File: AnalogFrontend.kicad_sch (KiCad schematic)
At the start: 6 parts, among them IC1 RMS-30+, IC2 SKY65405-21, J1 Conn_Coaxial_x2, J2 Conn_Coaxial_x2, J3 USB_A

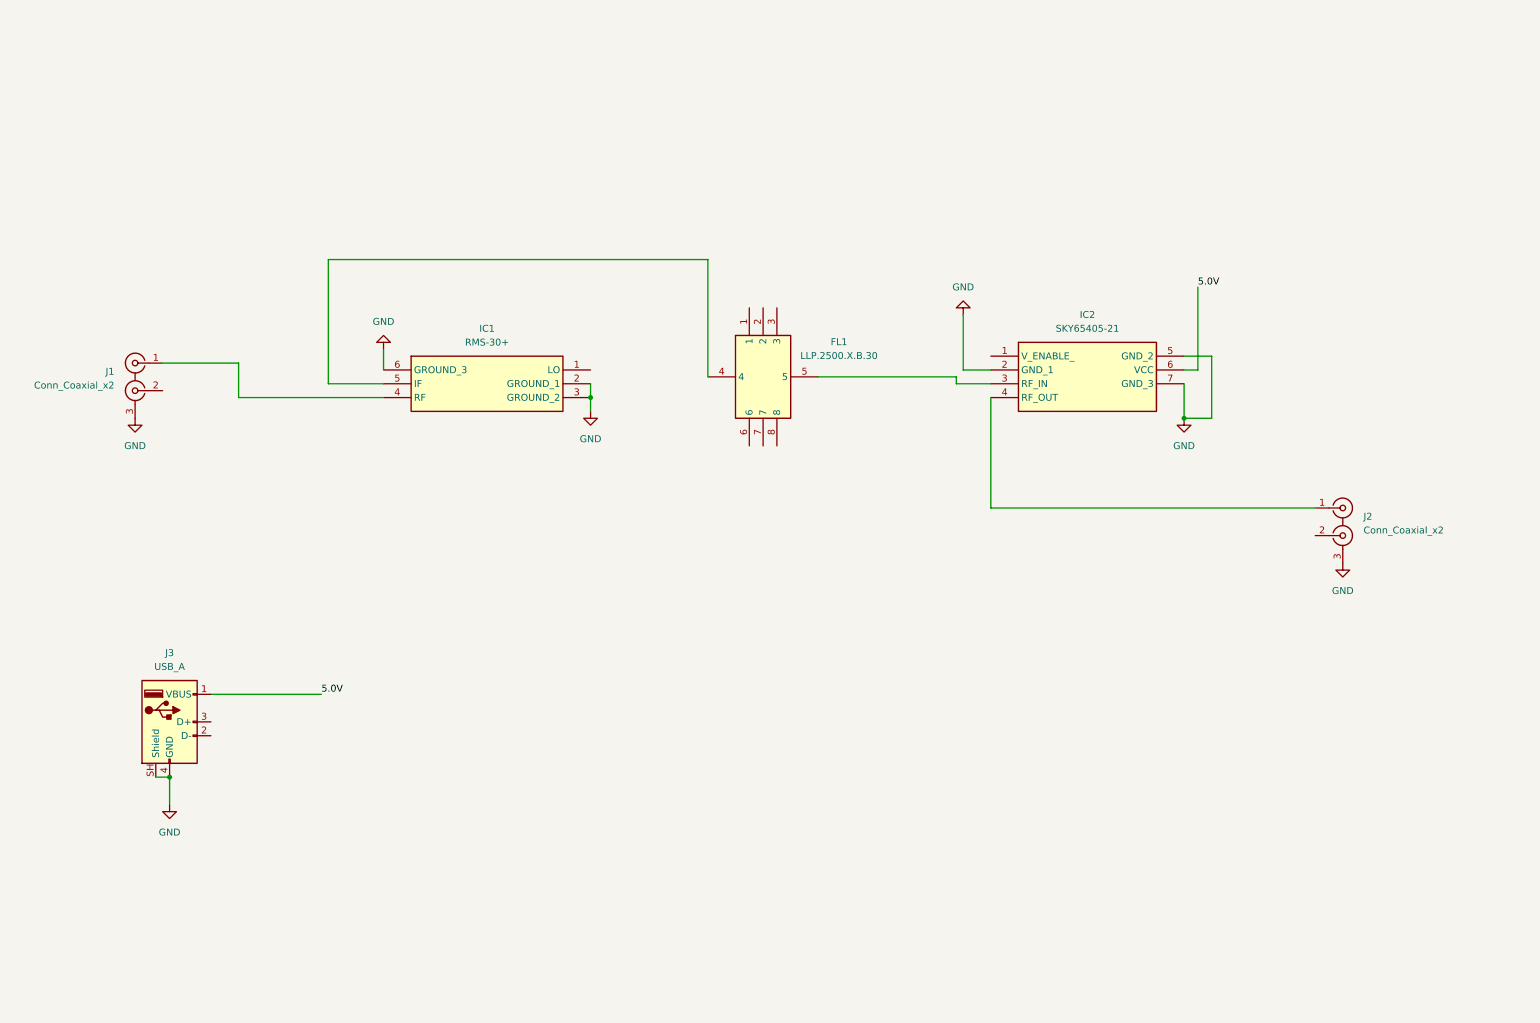
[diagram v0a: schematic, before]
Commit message: updatged schematics
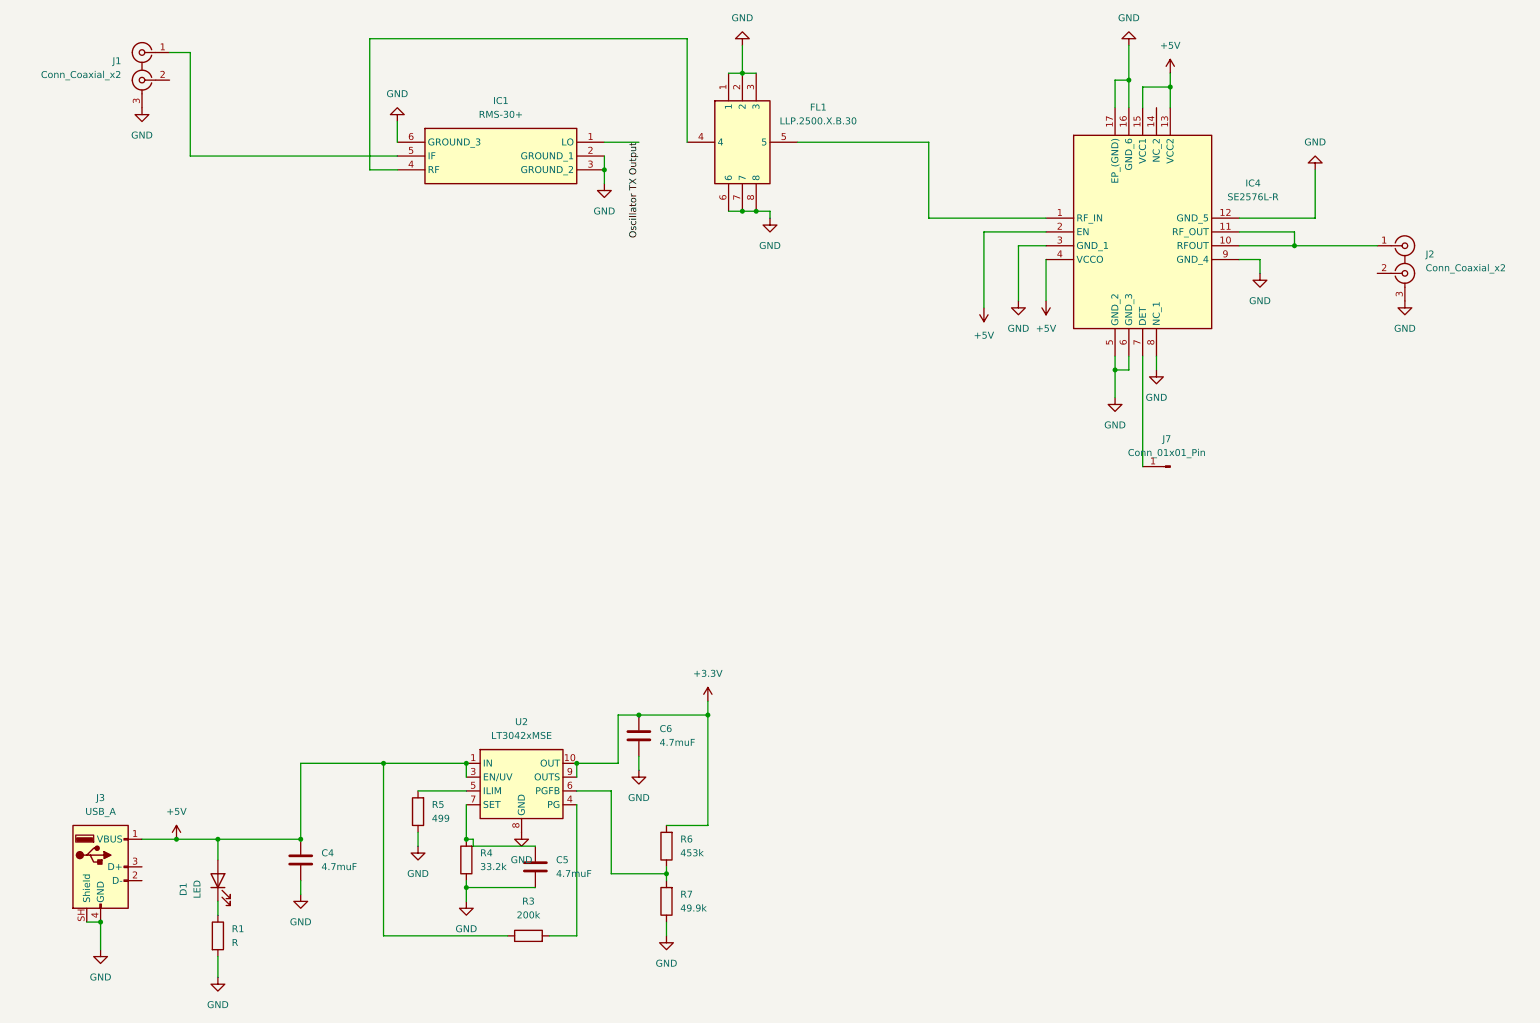
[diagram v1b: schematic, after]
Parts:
- removed IC2: SKY65405-21, SKY6540521, symbol SamacSys_Parts:SKY65405-21
- added C4, C5, C6: 4.7muF, Capacitor_SMD:C_1206_3216Metric_Pad1.33x1.80mm_HandSolder, symbol Device:C
- added D1: LED, symbol Device:LED
- added IC4: SE2576L-R, SamacSys_Parts:QFN50P300X300X90-17N-D, symbol SamacSys_Parts:SE2576L-R
- added J7: Conn_01x01_Pin, symbol Connector:Conn_01x01_Pin
- added R1: R, Resistor_SMD:R_0612_1632Metric_Pad1.18x3.40mm_HandSolder, symbol Device:R
- added R3: 200k, Resistor_SMD:R_0612_1632Metric_Pad1.18x3.40mm_HandSolder, symbol Device:R
- added R4: 33.2k, Resistor_SMD:R_0612_1632Metric_Pad1.18x3.40mm_HandSolder, symbol Device:R
- added R5: 499, Resistor_SMD:R_0612_1632Metric_Pad1.18x3.40mm_HandSolder, symbol Device:R
- added R6: 453k, Resistor_SMD:R_0612_1632Metric_Pad1.18x3.40mm_HandSolder, symbol Device:R
- added R7: 49.9k, Resistor_SMD:R_0612_1632Metric_Pad1.18x3.40mm_HandSolder, symbol Device:R
- added U2: LT3042xMSE, Package_SO:MSOP-10-1EP_3x3mm_P0.5mm_EP1.68x1.88mm, symbol Regulator_Linear:LT3042xMSE
- FL1: footprint LLP2500XB30 -> SamacSys_Parts:LLP2500XB30
- IC1: footprint RMS30 -> SamacSys_Parts:RMS30
- J3: footprint (none) -> Connector_USB:USB3_A_Molex_48393-001
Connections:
- net GND: now also FL1.1, FL1.2, FL1.3, FL1.6, FL1.7, FL1.8, C4.2, C5.2, C6.2, IC4.12 (GND_5), IC4.16 (GND_6), IC4.17 (EP_(GND)), IC4.3 (GND_1), IC4.5 (GND_2), IC4.6 (GND_3), IC4.8 (NC_1), IC4.9 (GND_4), R1.2, R4.1, R5.1, R7.1, U2.11 (GND), U2.8 (GND)
- net at J1.1 (IN1): now also IC1.5 (IF); no longer IC1.4 (RF)
- net at FL1.4: now also IC1.4 (RF); no longer IC1.5 (IF)
- net at FL1.5: now also IC4.1 (RF_IN)
- net Oscillator TX Output: now reaches IC1.1 (LO)
- net at J2.1 (IN1): now also IC4.10 (RFOUT), IC4.11 (RF_OUT)
- net 5.0V renamed +5V
- net +5V: now also C4.1, D1.2 (A), IC4.13 (VCC2), IC4.15 (VCC1), IC4.2 (EN), IC4.4 (VCCO), R3.1, U2.1 (IN), U2.2 (IN), U2.3 (EN/UV)
- new net: IC4.7 (DET), J7.1 (Pin_1)
- new net: R6.1, R7.2, U2.6 (PGFB)
- new net: D1.1 (K), R1.1
- new net: R3.2, U2.4 (PG)
- new net: R5.2, U2.5 (ILIM)
- new net: C5.1, R4.2, U2.7 (SET)
- new net +3.3V: C6.1, R6.2, U2.10 (OUT), U2.9 (OUTS)
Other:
- moved on the sheet: FL1, IC1, J1, J2, J3
